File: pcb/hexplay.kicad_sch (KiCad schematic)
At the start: 23 parts, among them J1 Conn_01x05_Pin, J2 Conn_01x05_Pin, SW1 SW_Push, SW10 SW_Push, SW11 SW_Push, SW12 SW_Push, SW13 SW_Push, SW14 SW_Push, SW15 SW_Push, SW2 SW_Push, SW3 SW_Push, SW4 SW_Push, SW5 SW_Push, SW6 SW_Push, SW7 SW_Push, SW8 SW_Push, SW9 SW_Push, U1 ADS7830

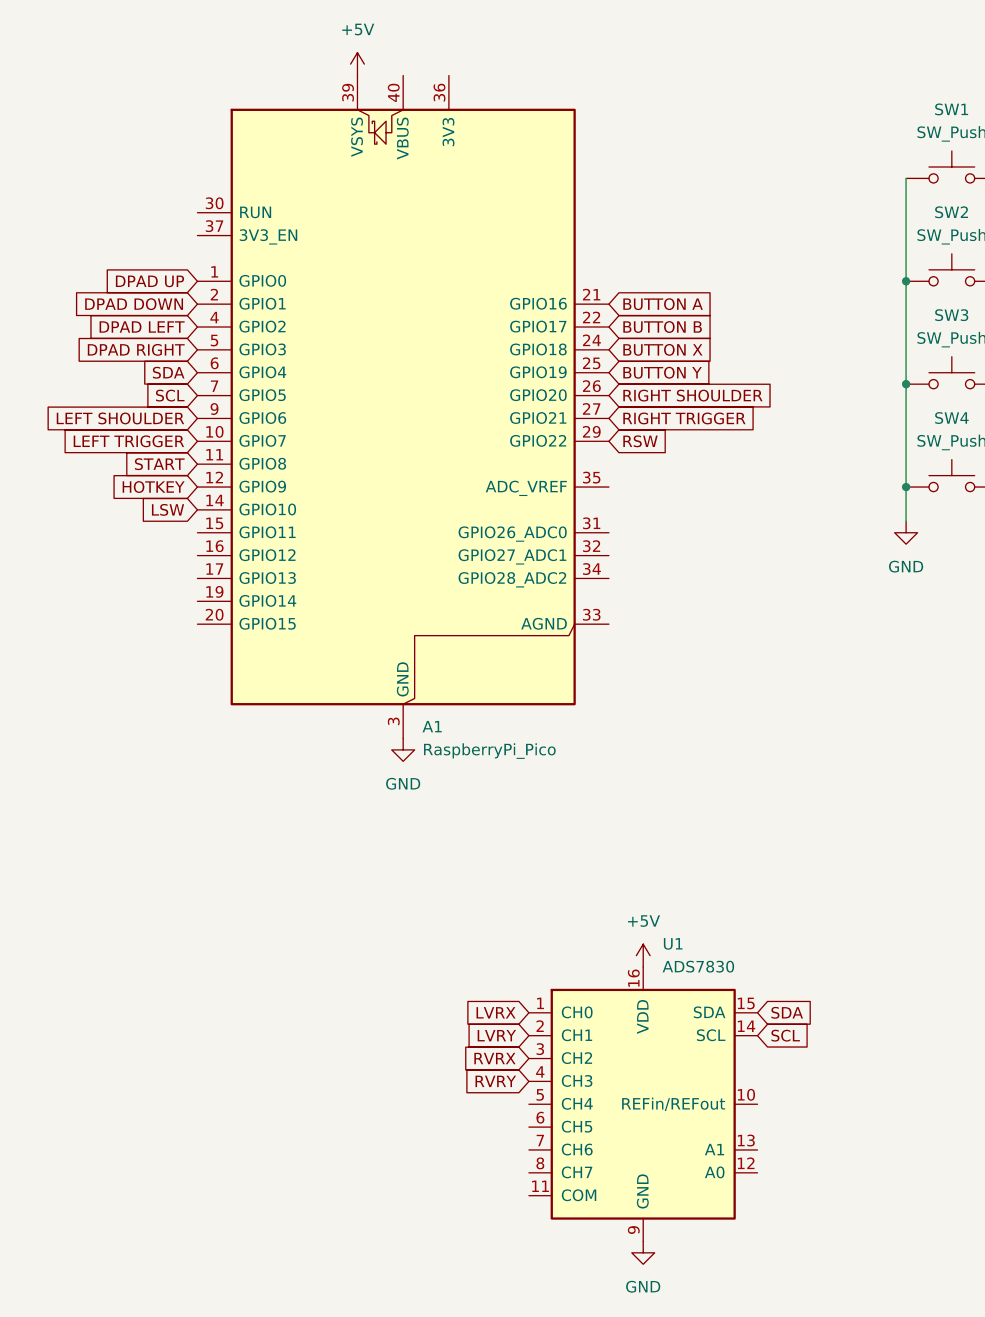
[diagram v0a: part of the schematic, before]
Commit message: added finalized cad files
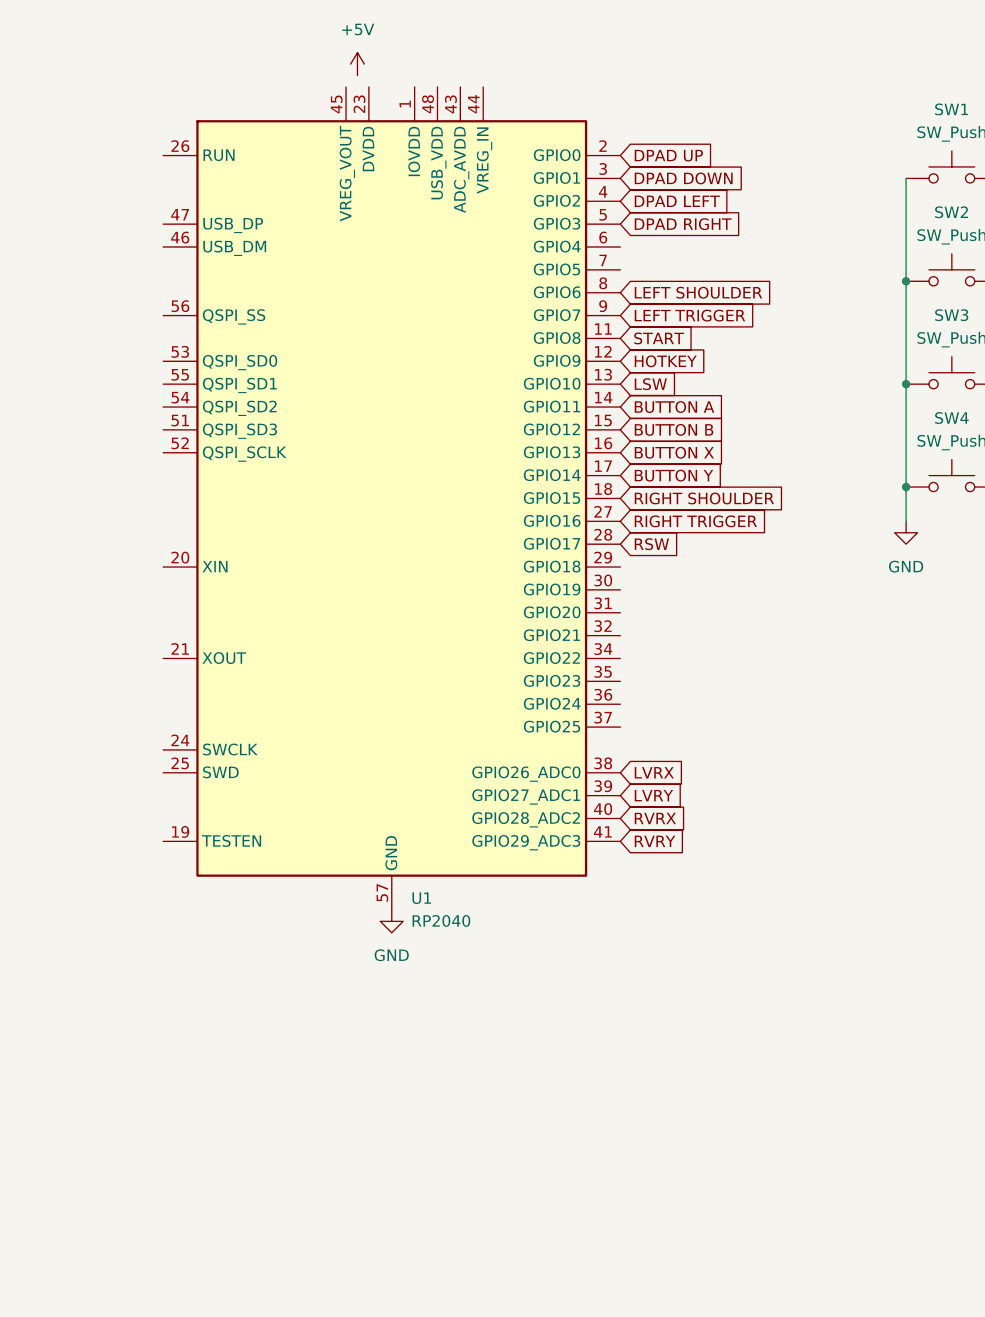
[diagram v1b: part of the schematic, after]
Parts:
- removed A1: RaspberryPi_Pico, Module:RaspberryPi_Pico_Common_Unspecified, symbol MCU_Module:RaspberryPi_Pico
- removed U1: ADS7830, Package_SO:TSSOP-16_4.4x5mm_P0.65mm, symbol Analog_DAC:ADS7830
- added U1: RP2040, Package_DFN_QFN:QFN-56-1EP_7x7mm_P0.4mm_EP3.2x3.2mm, symbol MCU_RaspberryPi:RP2040
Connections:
- net BUTTON A: now also U1.14 (GPIO11)
- net BUTTON B: now also U1.15 (GPIO12)
- net BUTTON X: now also U1.16 (GPIO13)
- net BUTTON Y: now also U1.17 (GPIO14)
- net DPAD DOWN: now also U1.3 (GPIO1)
- net DPAD LEFT: now also U1.4 (GPIO2)
- net DPAD RIGHT: now also U1.5 (GPIO3)
- net DPAD UP: now also U1.2 (GPIO0)
- net GND: now also U1.57 (GND)
- net HOTKEY: now also U1.12 (GPIO9)
- net LEFT SHOULDER: now also U1.8 (GPIO6)
- net LEFT TRIGGER: now also U1.9 (GPIO7)
- net LSW: now also U1.13 (GPIO10)
- net LVRX: now also U1.38 (GPIO26_ADC0)
- net LVRY: now also U1.39 (GPIO27_ADC1)
- net RIGHT SHOULDER: now also U1.18 (GPIO15)
- net RIGHT TRIGGER: now also U1.27 (GPIO16)
- net RSW: now also U1.28 (GPIO17)
- net RVRX: now also U1.40 (GPIO28_ADC2)
- net RVRY: now also U1.41 (GPIO29_ADC3)
- net START: now also U1.11 (GPIO8)
- net at MP1. (ETHERNET): now also DS1. (HDMI)
- new net: U1.1 (IOVDD), U1.10 (IOVDD), U1.22 (IOVDD), U1.33 (IOVDD), U1.42 (IOVDD), U1.49 (IOVDD)
- new net: U1.23 (DVDD), U1.50 (DVDD)
- new net: DS1. (HDMI), MP1. (ETHERNET)
